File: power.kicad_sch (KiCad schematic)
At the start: 32 parts, among them IC1 TPS630702RNMR, IC2 RT6150B-33GQW, J1 USB_C_Receptacle_USB2.0_16P, J8 1053141104, U5 MG6206K3B

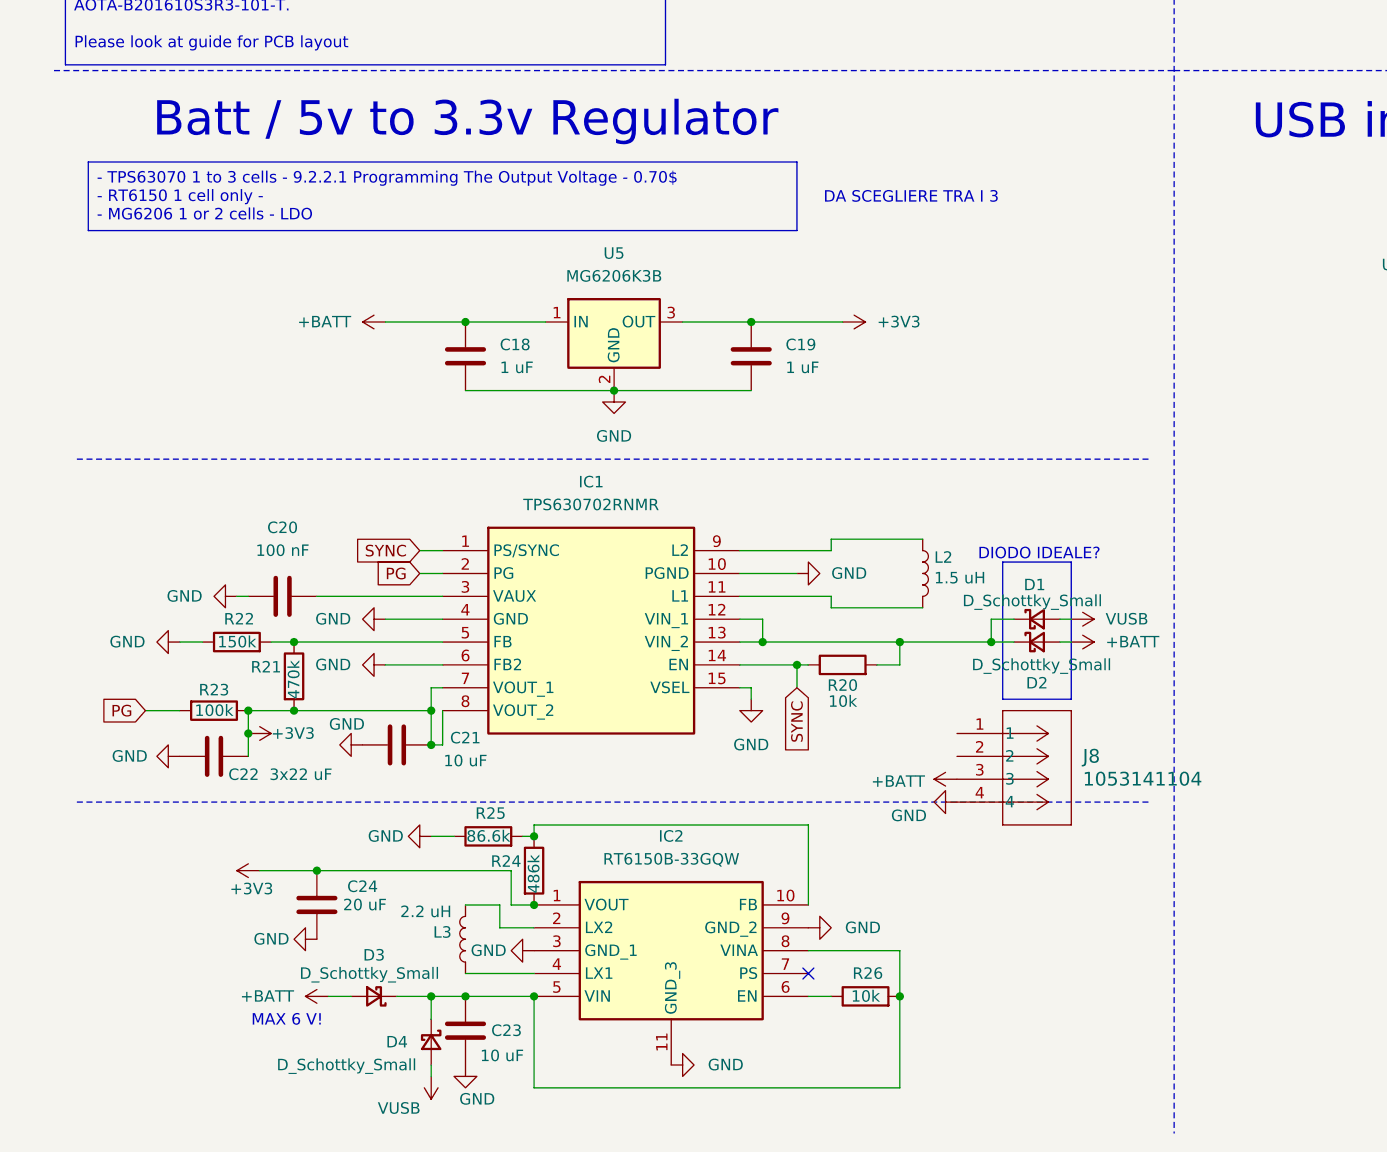
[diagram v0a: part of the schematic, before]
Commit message: changes 20/12
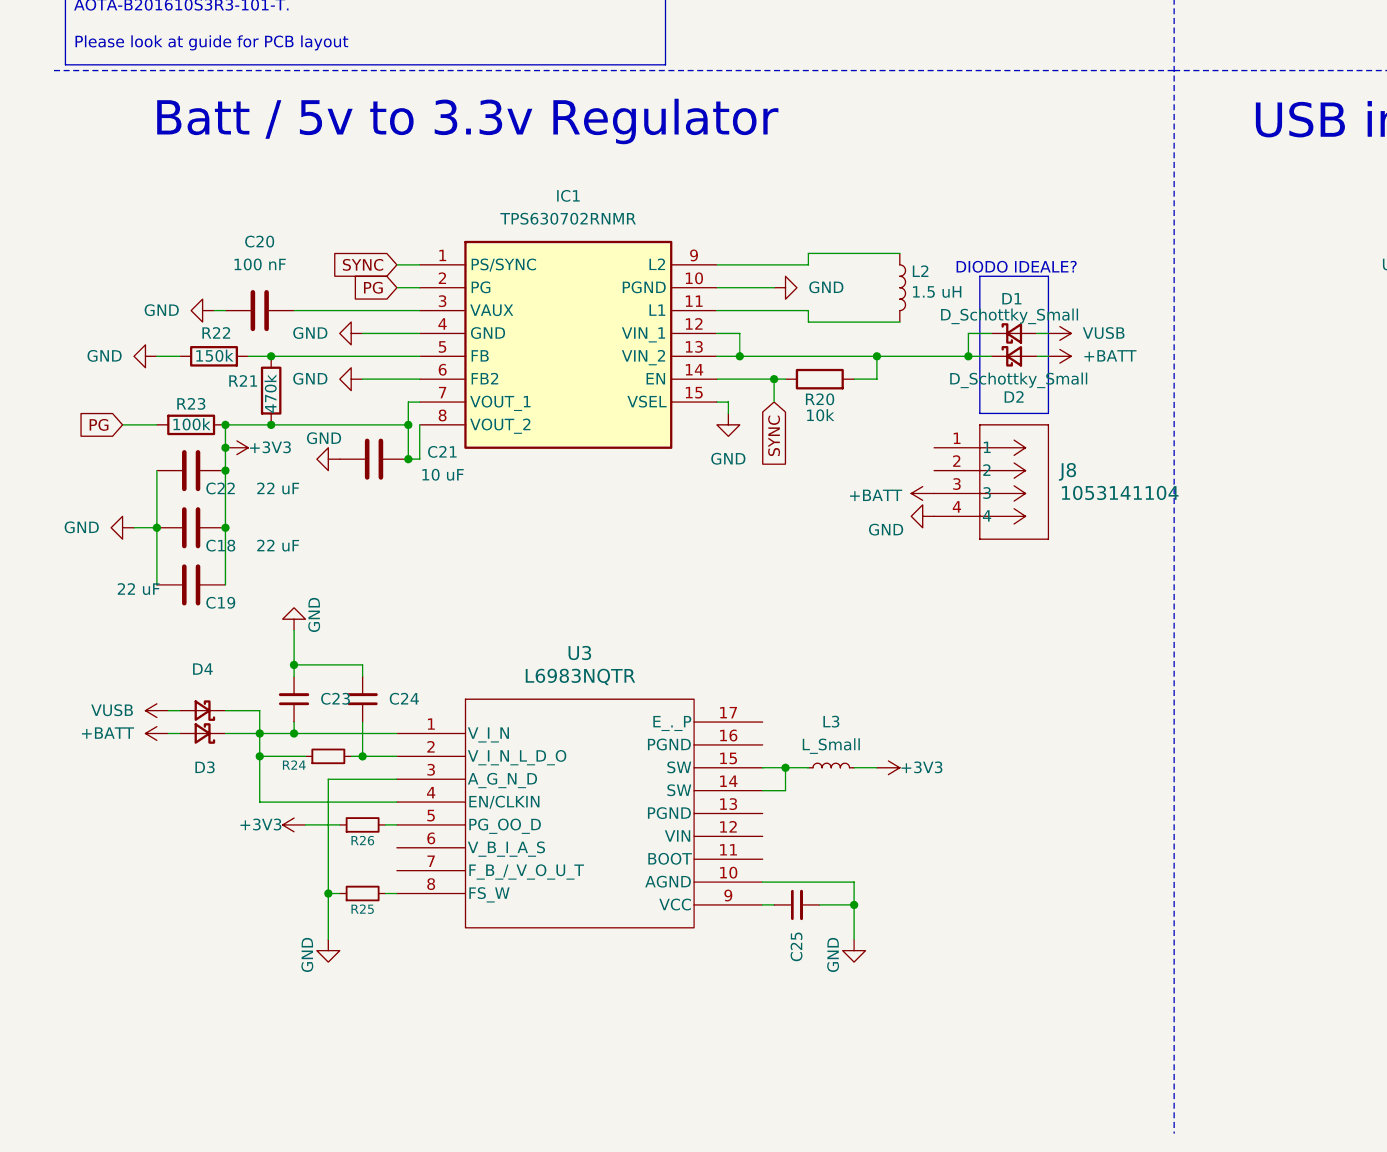
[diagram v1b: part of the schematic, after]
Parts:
- removed C23: 10 uF, symbol Device:C
- removed C24: 20 uF, symbol Device:C
- removed IC2: RT6150B-33GQW, SON50P250X250X80-11N-D, symbol RT6150B-33GQW:RT6150B-33GQW
- removed L3: 2.2 uH, symbol Device:L
- removed R24: 486k, symbol Device:R
- removed R25: 86.6k, symbol Device:R
- removed R26: 10k, symbol Device:R
- removed U5: MG6206K3B, Package_TO_SOT_SMD:TSOT-23_HandSoldering, symbol Regulator_Linear:UA78M33QDCYRQ1
- added C23, C24, C25: C_Small, symbol Device:C_Small
- added L3: L_Small, symbol Device:L_Small
- added R24, R25, R26: R_Small, symbol Device:R_Small
- added U3: L6983NQTR, QFN_NQTR_STM, symbol 2025-12-20_10-01-49:L6983NQTR
- C18, C19: value 1 uF -> 22 uF; footprint (none) -> Capacitor_SMD:C_0603_1608Metric_Pad1.08x0.95mm_HandSolder; now in the parts list
- C22: value 3x22 uF -> 22 uF
- D3, D4: footprint (none) -> SDM2U30CSP:SDM2U30CSP; now in the parts list
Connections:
- net +3V3: now also C18.1, L3.2, R26.1
- net +BATT: no longer C18.1
- net GND: now also C23.2, C24.2, C25.2, R25.1, U3.10 (AGND), U3.3 (A_G_N_D)
- net at D3.1 (K), D4.1 (K): now also C23.1, R24.1, U3.1 (V_I_N), U3.4 (EN/CLKIN)
- new net: L3.1, U3.14 (SW), U3.15 (SW)
- new net: C24.1, R24.2, U3.2 (V_I_N_L_D_O)
- new net: R26.2, U3.5 (PG_OO_D)
- new net: R25.2, U3.8 (FS_W)
- new net: C25.1, U3.9 (VCC)
- no-connect marks 5 -> 4
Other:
- note removed: "DA SCEGLIERE TRA I 3"
- note removed: "MAX 6 V!"
- moved on the sheet: C20, C21, C22, D1, D2, IC1, J8, L2, R20, R21, R22, R23
